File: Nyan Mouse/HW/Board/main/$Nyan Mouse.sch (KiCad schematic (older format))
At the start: 35 parts, among them M101 BATTBALANCE-2S, P101 Controller Connector, P102 CONN_4, P103 CONN_2, P104 CONN_2, P105 motor_a, P106 motor_b, U101 DRV8837, U102 DRV8837

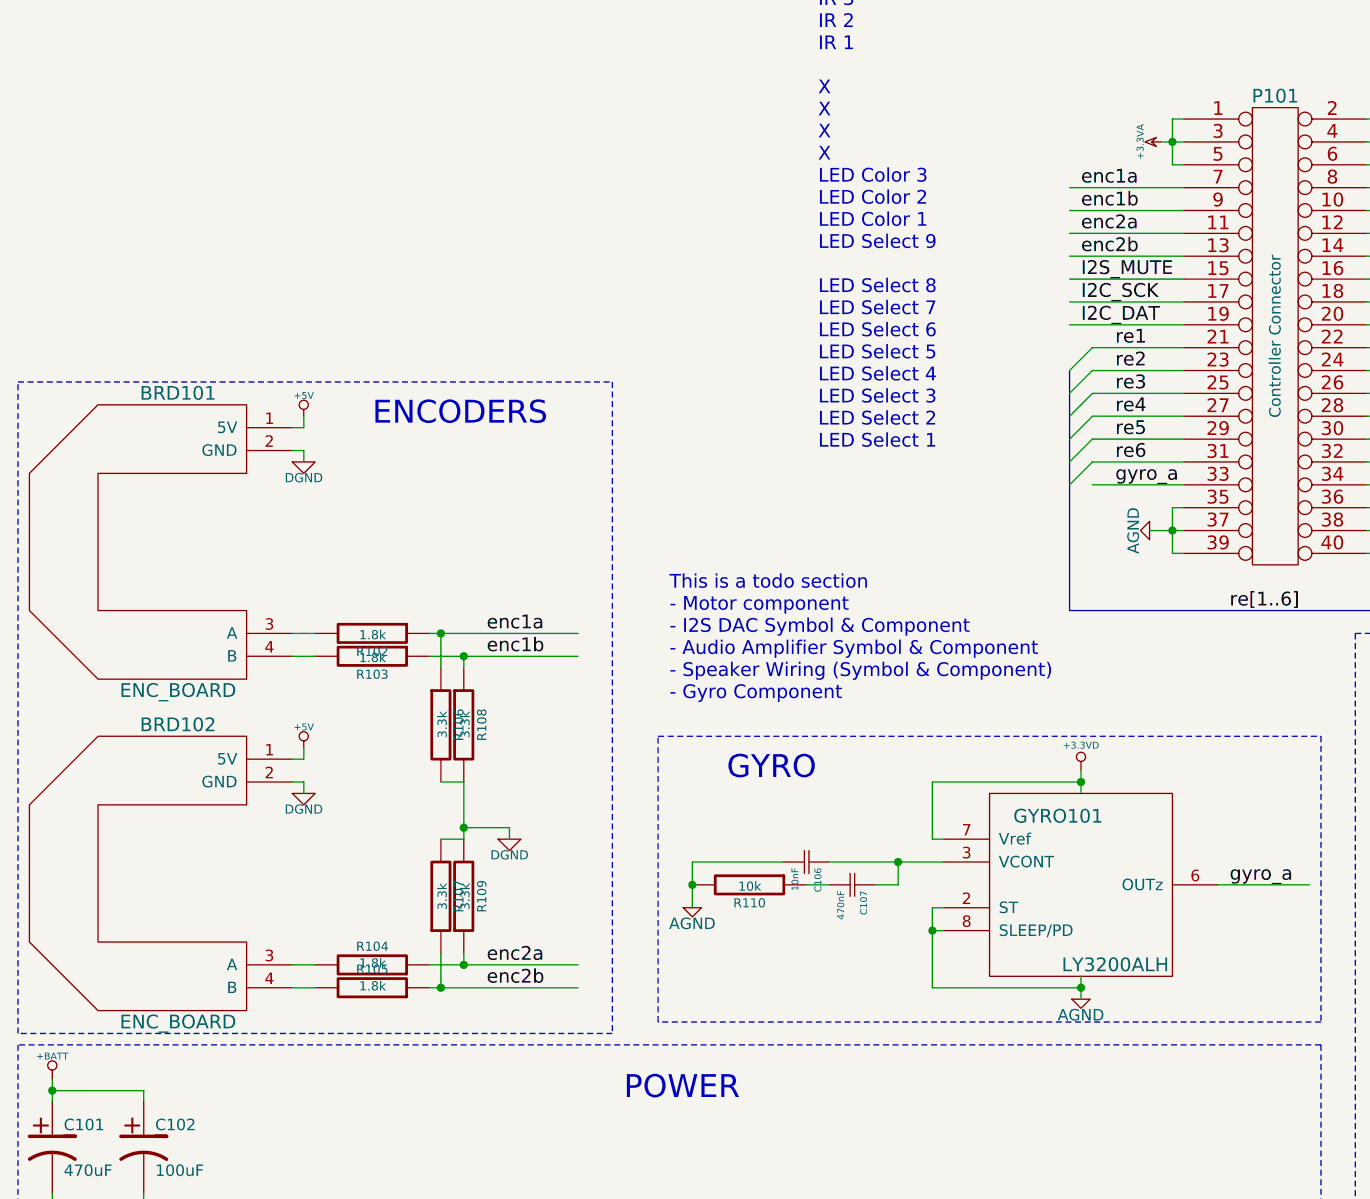
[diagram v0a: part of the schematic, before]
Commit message: Updated schematics
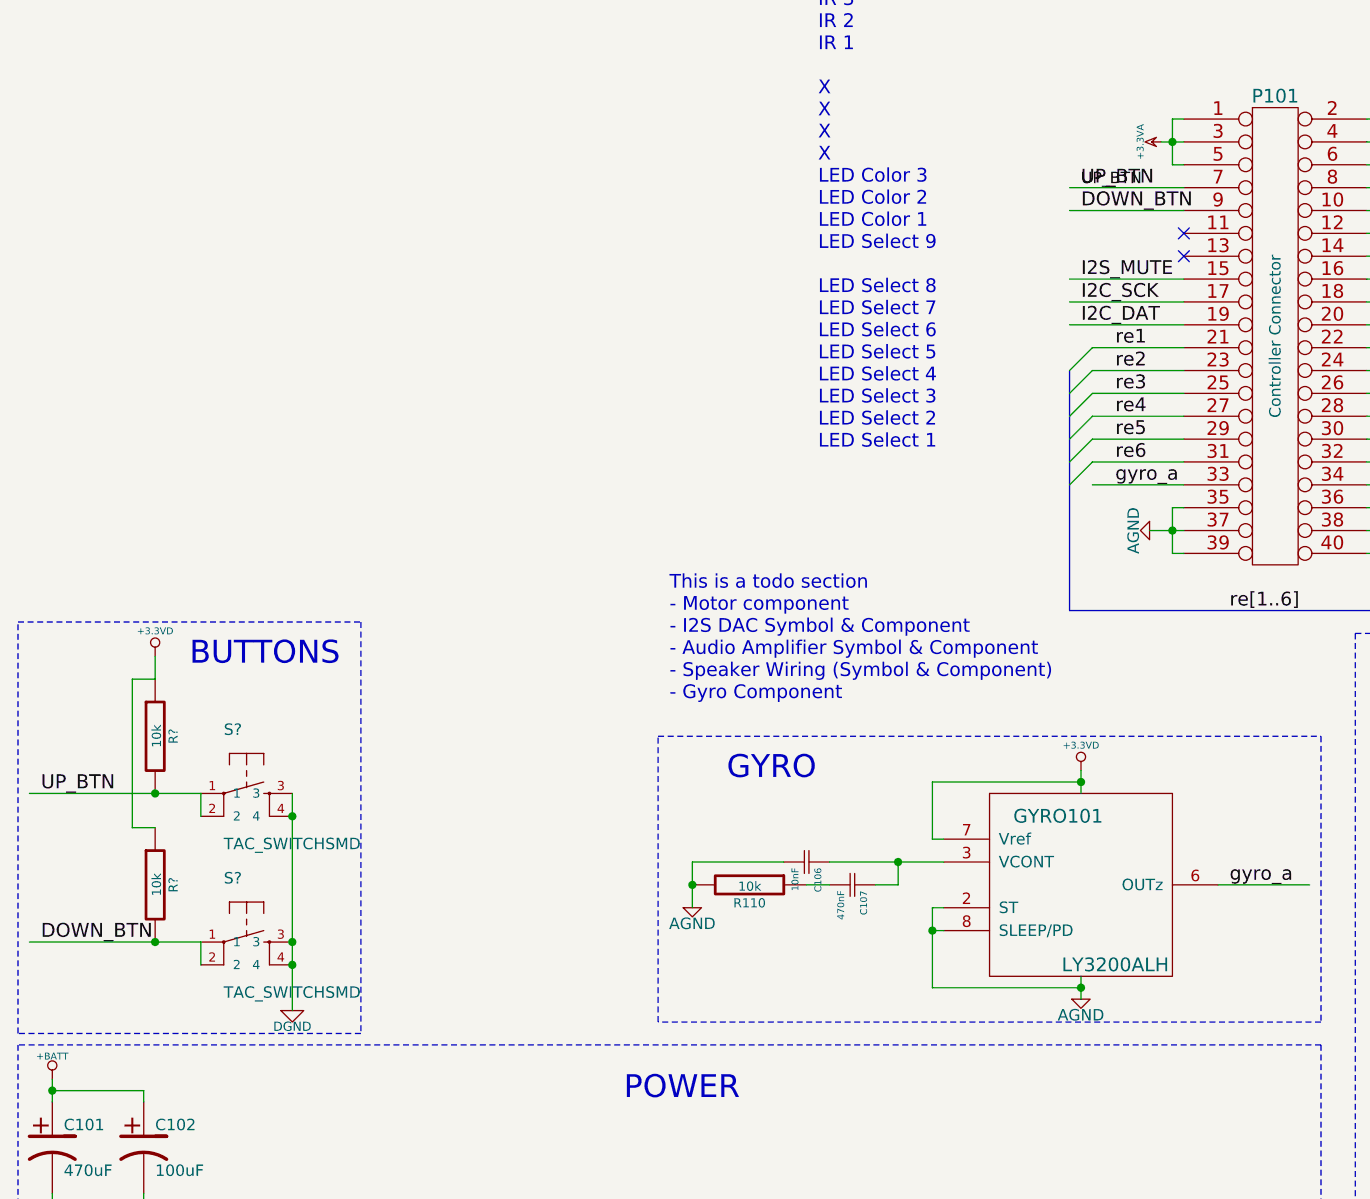
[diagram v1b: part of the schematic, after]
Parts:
- removed BRD101, BRD102: ENC_BOARD, symbol ENC_BOARD
- removed R102, R103, R104, R105: 1.8k, symbol R
- removed R106, R107, R108, R109: 3.3k, symbol R
- added R? (x2): 10k, symbol R
- added S? (x2): TAC_SWITCHSMD, SparkFun-TACTILE_SWITCH_SMD, symbol TAC_SWITCHSMD
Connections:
- net labels added: DOWN_BTN, UP_BTN
- net labels removed: enc1a, enc1b, enc2a, enc2b
- wire segments 195 -> 177
- no-connect marks 1 -> 3
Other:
- note added: "BUTTONS"
- note removed: "ENCODERS"
